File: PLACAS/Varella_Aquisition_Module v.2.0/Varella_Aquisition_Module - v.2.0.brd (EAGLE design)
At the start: 100 x 80 mm, 62 parts, among them IC1 M95M04-DRDW6TP, IC10 ICL7660SCBAZ, IC3 M95M04-DRDW6TP, IC4 M95M04-DRDW6TP, IC9 M95M04-DRDW6TP, U1 FT232RLSSOP, X2 USB-SMD-NS, Y2 FA-20H_16.0000MF10Z-AJ0

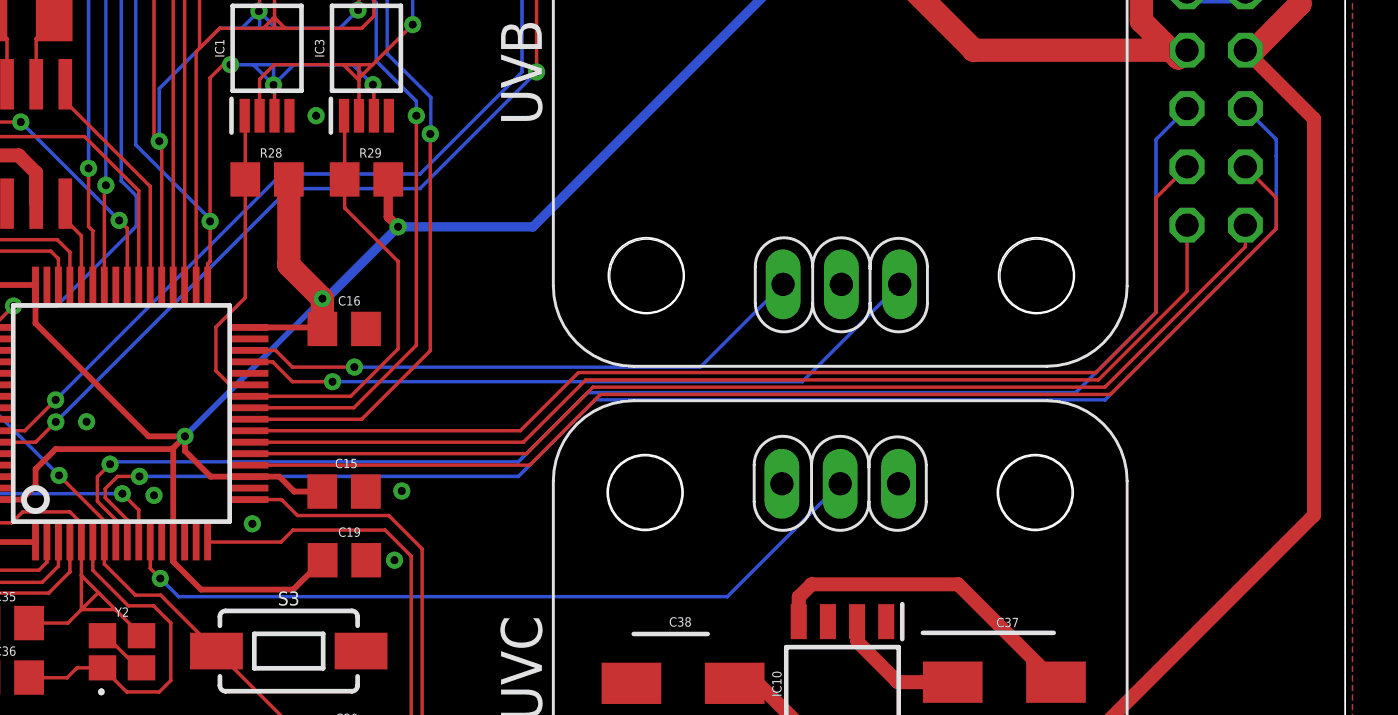
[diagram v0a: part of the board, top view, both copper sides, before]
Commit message: Add files via upload
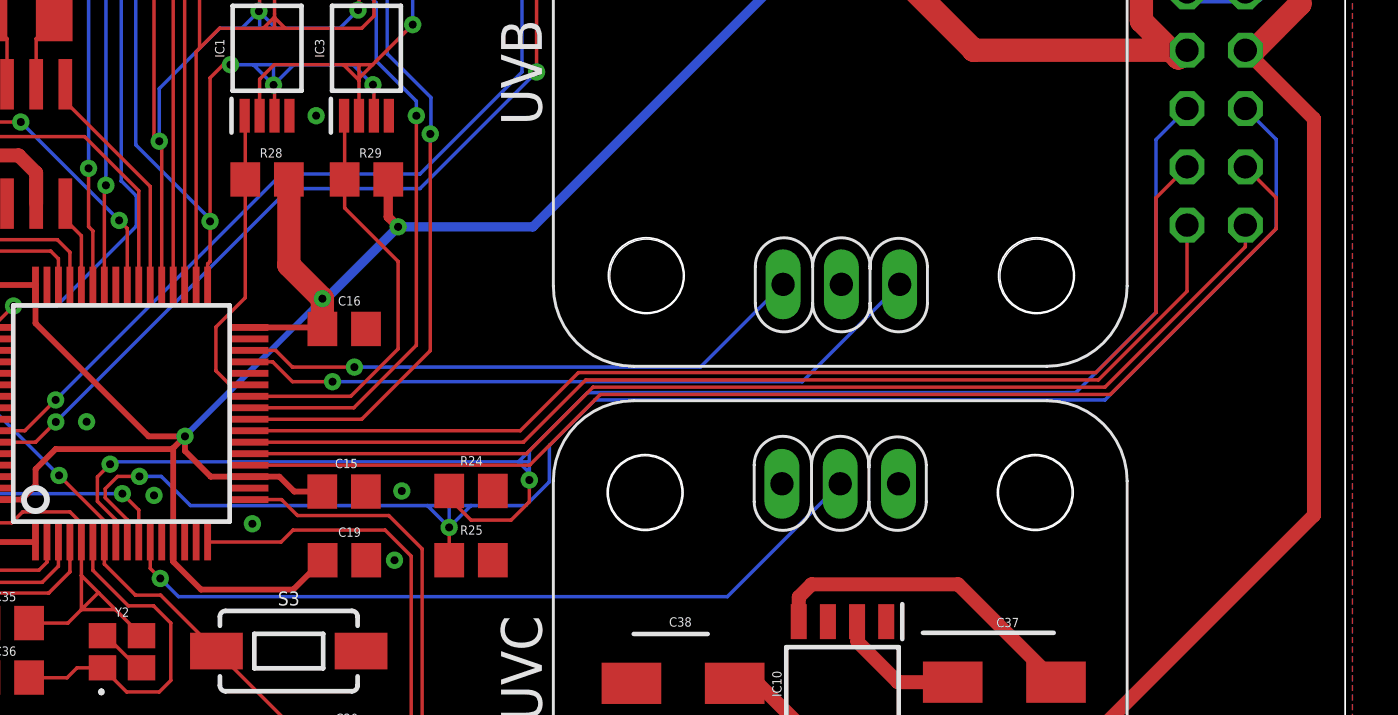
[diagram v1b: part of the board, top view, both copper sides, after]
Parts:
- added R24, R25: 4,7k, rcl:R0805
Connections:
- net +3V3: now also R24.2, R25.2
- net SCL3: now also R24.1
- net SDA3: now also R25.1
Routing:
- net SCL3: track 61.7 -> 69.6 mm, vias 1 -> 2
- net SDA3: track 64.2 -> 71.3 mm, vias 1 -> 2
